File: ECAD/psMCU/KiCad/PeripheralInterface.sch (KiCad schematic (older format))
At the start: 32 parts, among them J6 PERIPH_INTERFACE, U26 SN74HC245PW, U27 SN74HC245PW, U28 SN74LVC1G86DCK, U29 SN74HC245PW, U30 SN74LVC1G04DCK, U349 SN74LVC1G08DCK, U350 SN74LVC1G08DCK, U351 SN74LVC1G08DCK, U437 SN74LVC1G08DCK, U438 SN74LVC1G08DCK, U439 SN74LVC1G32DCK, U440 SN74LVC1G32DCK, U441 SN74LVC1G126DCK

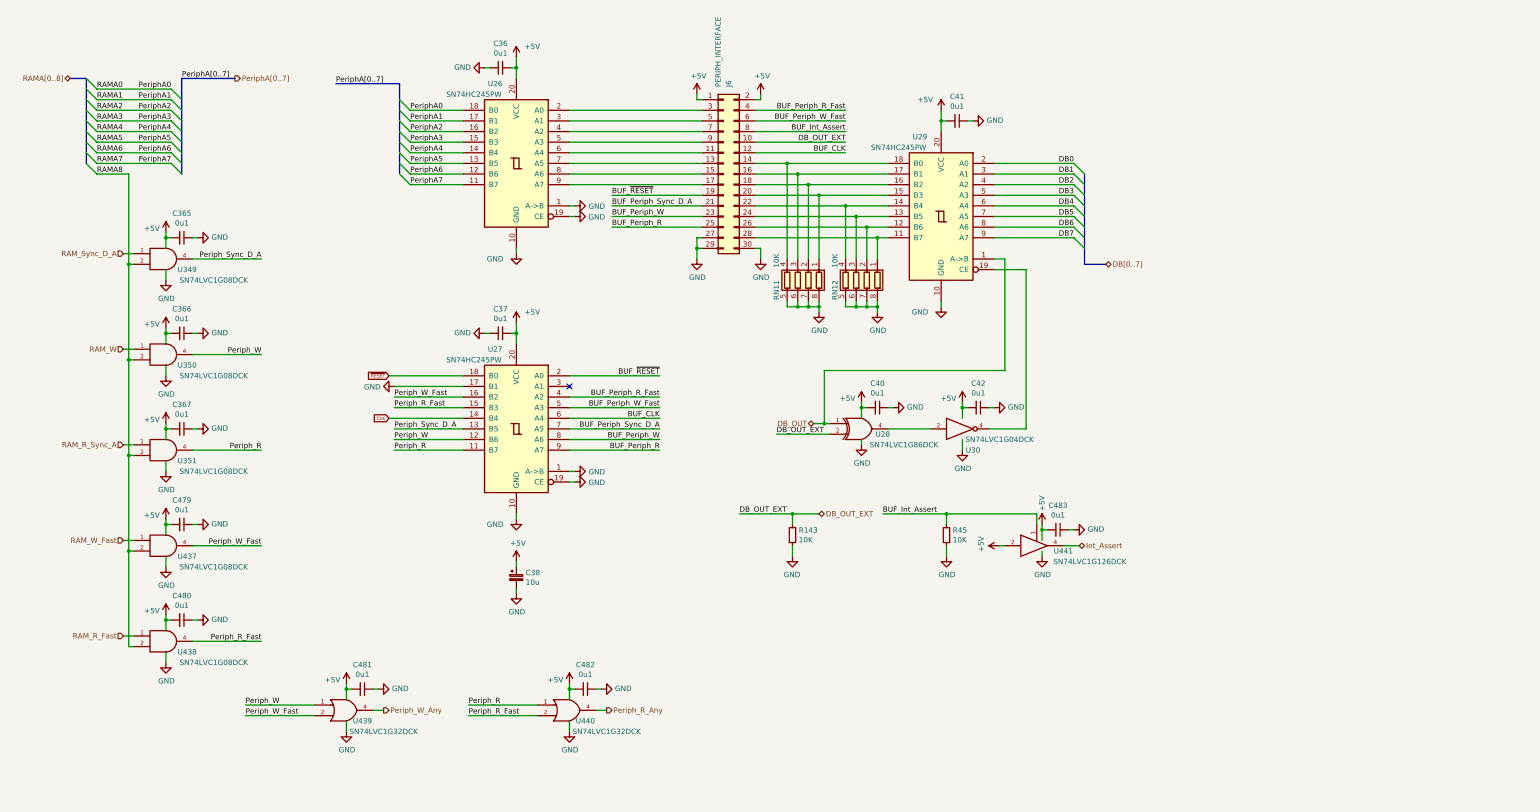
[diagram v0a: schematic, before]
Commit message: Sch: Cleanup + Small fixes
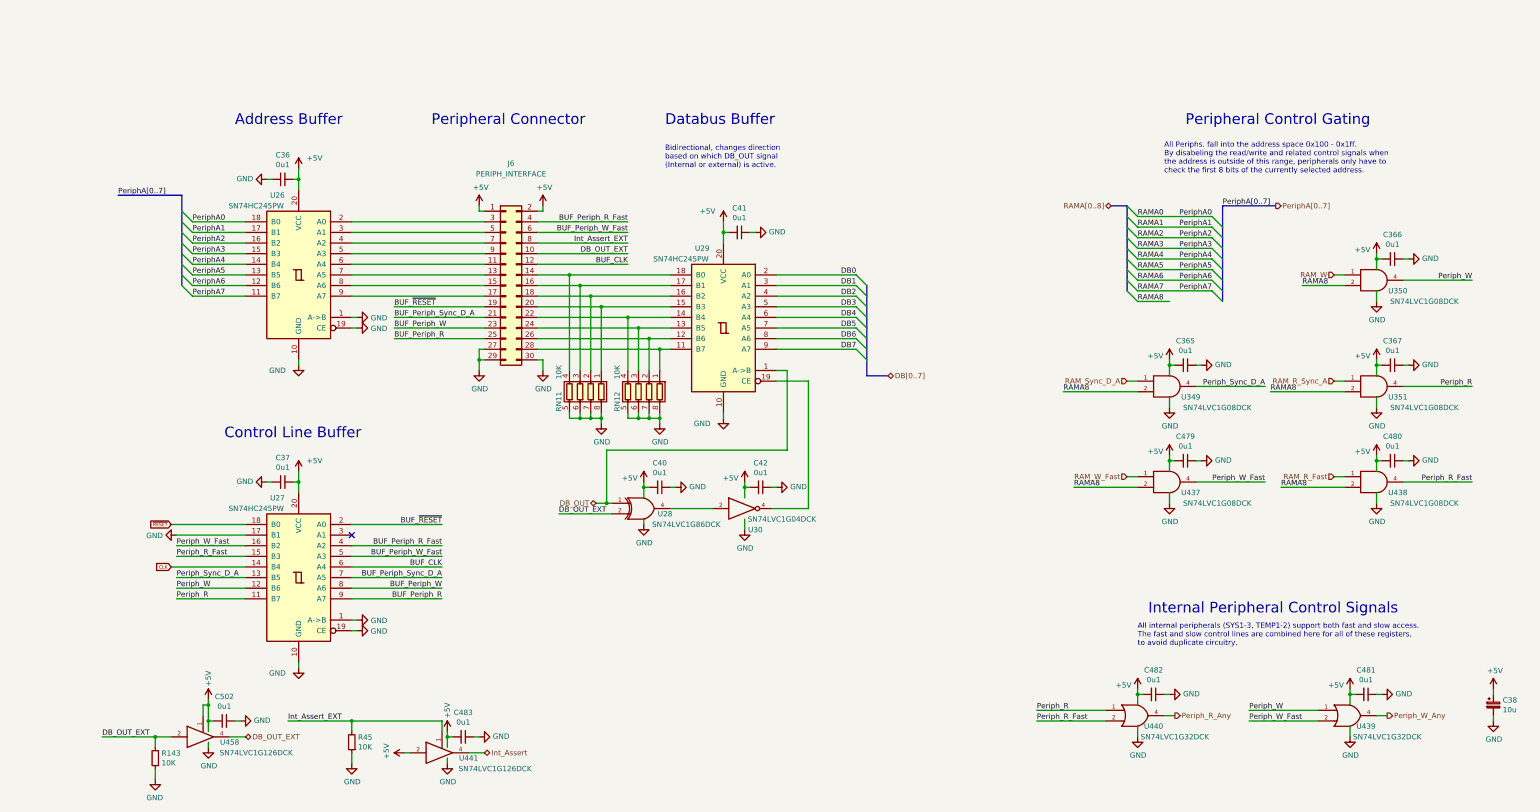
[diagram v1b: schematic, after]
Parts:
- added C502: 0u1, NoRef_Footprints:C_0603_1608Metric_NoRef, symbol Device:C_Small
- added U458: SN74LVC1G126DCK, Package_TO_SOT_SMD:SOT-353_SC-70-5, symbol 74xGxx:74LVC1G126
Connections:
- net +5V: now also C502.2, U458.1, U458.5 (VCC)
- net DB_OUT_EXT: now also U458.2, U458.4
- net GND: now also C502.1, U458.3 (GND)
- net BUF_Int_Assert renamed Int_Assert_EXT
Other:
- note added: "Address Buffer"
- note added: "All Periphs. fall into the address space 0x100 - 0x1ff.\nBy disabeling the read/write and related control signals when\nthe address is outside of this range, peripherals only have to\ncheck the first 8 bits of the currently selected address."
- note added: "All internal peripherals (SYS1-3, TEMP1-2) support both fast and slow access.\nThe fast and slow control lines are combined here for all of these registers, \nto avoid duplicate circuitry."
- note added: "Bidirectional, changes direction \nbased on which DB_OUT signal \n(Internal or external) is active."
- note added: "Control Line Buffer"
- note added: "Databus Buffer"
- note added: "Internal Peripheral Control Signals"
- note added: "Peripheral Connector"
- note added: "Peripheral Control Gating"
- moved on the sheet: C36, C365, C366, C367, C37, C38, C40, C41, C42, C479, C480, C481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
